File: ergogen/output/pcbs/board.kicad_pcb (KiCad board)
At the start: 2 copper layers, 155.7 x 107.9 mm, 58 parts

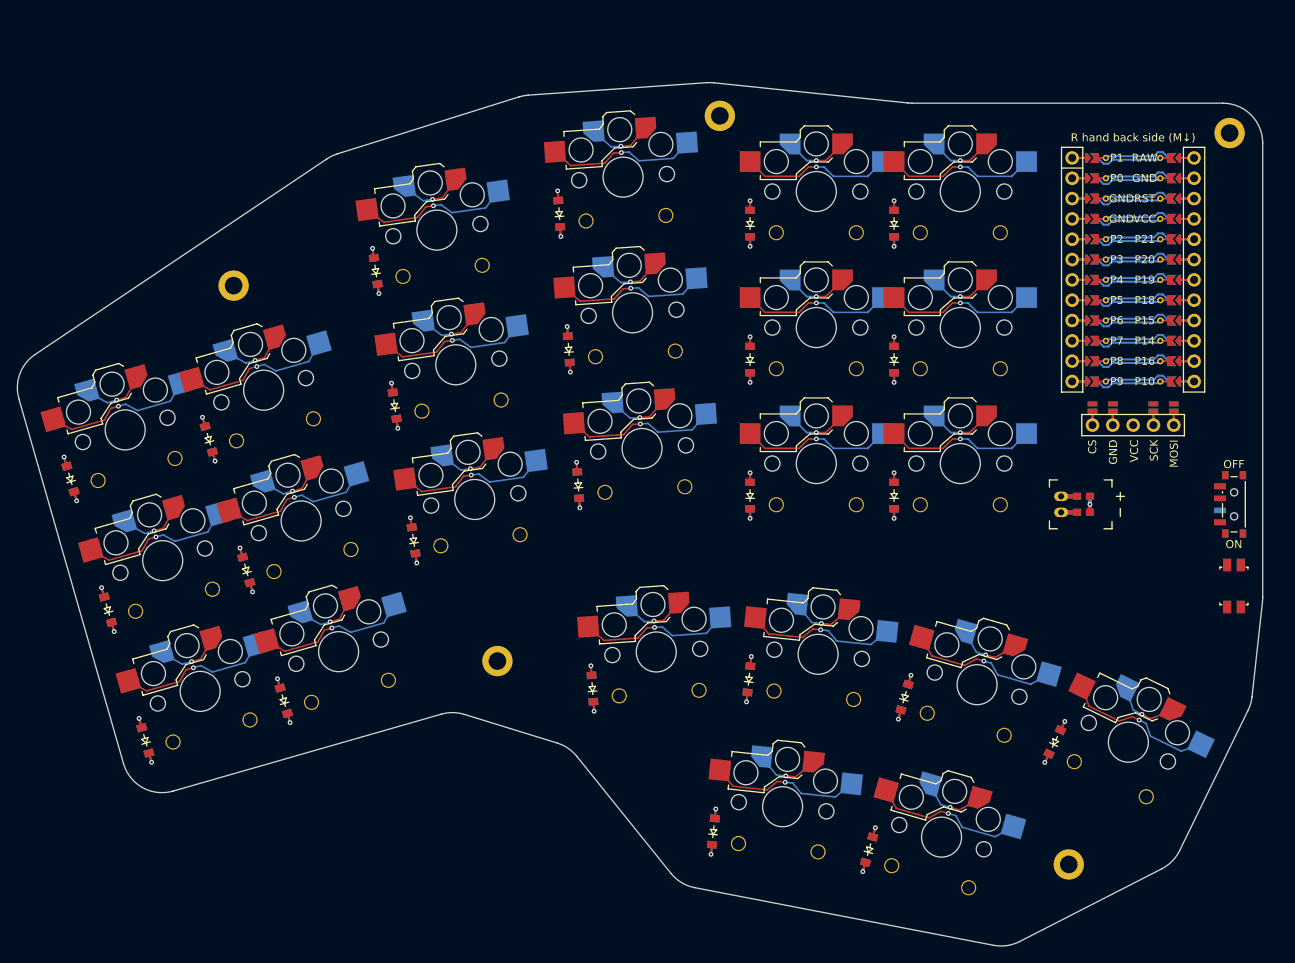
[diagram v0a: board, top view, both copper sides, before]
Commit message: moved the keys around as desired
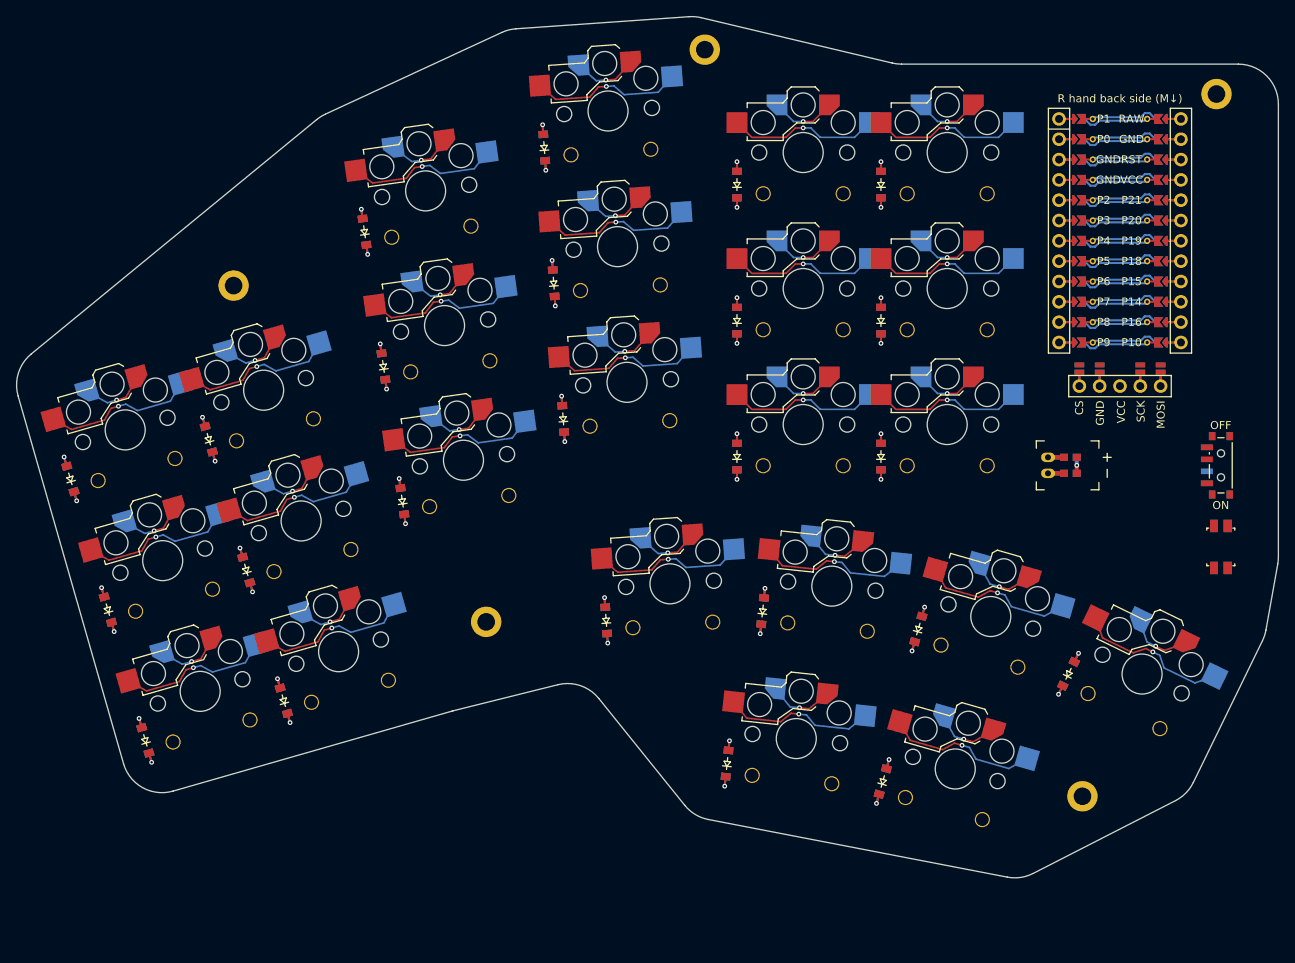
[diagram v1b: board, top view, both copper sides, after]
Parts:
- moved D22 8.69 mm to (258.5, 147.8)
- moved D19 8.69 mm to (200.7, 141.1)
- moved D20 8.69 mm to (220.3, 140.0)
- moved D21 8.69 mm to (239.8, 142.2)
- moved D23 8.69 mm to (215.9, 159.0)
- moved D24 8.69 mm to (235.3, 161.3)
- moved H4 8.69 mm to (260.3, 163.1)
- moved S19 8.69 mm to (208.7, 136.6)
- moved S20 8.69 mm to (229.0, 136.8)
- moved S21 8.69 mm to (248.8, 140.6)
- moved S22 8.69 mm to (267.7, 147.8)
- moved S23 8.69 mm to (224.5, 155.9)
- moved S24 8.69 mm to (244.4, 159.7)
- moved D10 8.48 mm to (195.4, 115.9)
- moved D11 8.48 mm to (194.2, 99.0)
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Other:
- board size 155.7 x 107.9 mm -> 157.7 x 107.7 mm
